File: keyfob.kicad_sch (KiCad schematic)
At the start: 6 parts, among them U1 ATtiny85V-10S

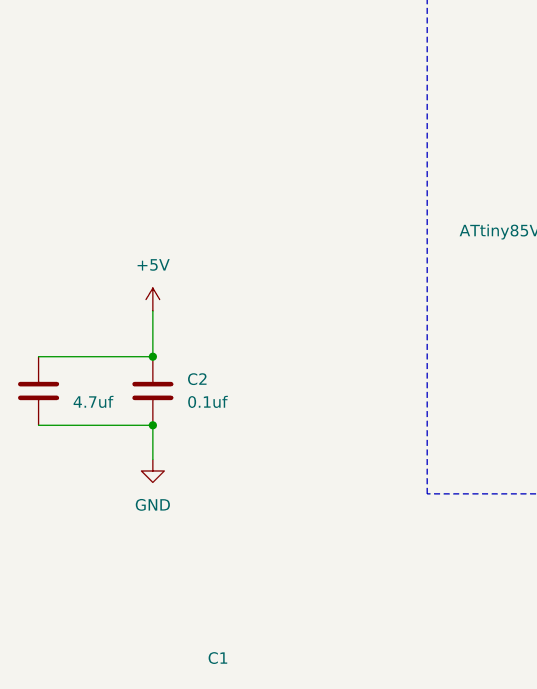
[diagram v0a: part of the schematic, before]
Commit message: Initial commit
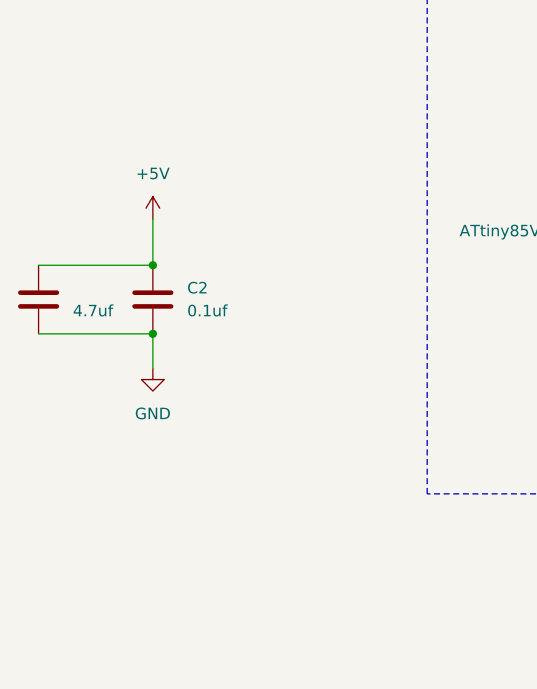
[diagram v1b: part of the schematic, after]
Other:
- moved on the sheet: C2
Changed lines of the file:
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@@
 	(paper "A4")
 	(junction
-		(at 142.24 113.03)
+		(at 142.24 102.87)
 		(diameter 0)
 		(color 0 0 0 0)
 	)
 	(junction
-		(at 142.24 120.65)
+		(at 142.24 110.49)
 		(diameter 0)
 		(color 0 0 0 0)
@@
 	(wire
 		(pts
-			(xy 129.54 113.03) (xy 142.24 113.03)
+			(xy 129.54 102.87) (xy 142.24 102.87)
 		)
 		(stroke
@@
 	(wire
 		(pts
-			(xy 142.24 107.95) (xy 142.24 113.03)
+			(xy 142.24 97.79) (xy 142.24 102.87)
 		)
 		(stroke
@@
 	(wire
 		(pts
-			(xy 129.54 120.65) (xy 142.24 120.65)
+			(xy 129.54 110.49) (xy 142.24 110.49)
 		)
 		(stroke
@@
 	(wire
 		(pts
-			(xy 142.24 120.65) (xy 142.24 124.46)
+			(xy 142.24 110.49) (xy 142.24 114.3)
 		)
 		(stroke
@@
 	(symbol
 		(lib_id "Device:C")
-		(at 129.54 116.84 0)
+		(at 129.54 106.68 0)
 		(unit 1)
 		(exclude_from_sim no)
@@
 		(dnp no)
 		(property "Reference" "C1"
-			(at 148.336 146.558 0)
+			(at 148.844 135.382 0)
 			(effects
 				(font
@@
 				)
 				(justify left)
+				(hide yes)
 			)
 		)
 		(property "Value" "4.7uf"
-			(at 133.35 118.1099 0)
+			(at 133.35 107.9499 0)
 			(effects
 				(font
@@
 		)
 		(property "Footprint" ""
-			(at 130.5052 120.65 0)
+			(at 130.5052 110.49 0)
 			(effects
 				(font
@@
 		)
 		(property "Datasheet" "~"
-			(at 129.54 116.84 0)
+			(at 129.54 106.68 0)
 			(effects
 				(font
@@
 		)
 		(property "Description" "Unpolarized capacitor"
-			(at 129.54 116.84 0)
+			(at 129.54 106.68 0)
 			(effects
 				(font
@@
 	(symbol
 		(lib_id "power:VCC")
-		(at 142.24 107.95 0)
+		(at 142.24 97.79 0)
 		(unit 1)
 		(exclude_from_sim no)
@@
 		(fields_autoplaced yes)
 		(property "Reference" "#PWR01"
-			(at 142.24 111.76 0)
+			(at 142.24 101.6 0)
 			(effects
 				(font
@@
 		)
 		(property "Value" "+5V"
-			(at 142.24 102.87 0)
-			(effects
-				(font
-					(size 1.27 1.27)
-				)
-			)
-		)
-		(property "Footprint" ""
-			(at 142.24 107.95 0)
+			(at 142.24 92.71 0)
+			(effects
+				(font
+					(size 1.27 1.27)
+				)
+			)
+		)
+		(property "Footprint" ""
+			(at 142.24 97.79 0)
 			(effects
 				(font
@@
 		)
 		(property "Datasheet" ""
-			(at 142.24 107.95 0)
+			(at 142.24 97.79 0)
 			(effects
 				(font
@@
 		)
 		(property "Description" "Power symbol creates a global label with name \"VCC\""
-			(at 142.24 107.95 0)
+			(at 142.24 97.79 0)
 			(effects
 				(font
@@
 	(symbol
 		(lib_id "power:GND")
-		(at 142.24 124.46 0)
+		(at 142.24 114.3 0)
 		(unit 1)
 		(exclude_from_sim no)
@@
 		(fields_autoplaced yes)
 		(property "Reference" "#PWR02"
-			(at 142.24 130.81 0)
+			(at 142.24 120.65 0)
 			(effects
 				(font
@@
 		)
 		(property "Value" "GND"
-			(at 142.24 129.54 0)
-			(effects
-				(font
-					(size 1.27 1.27)
-				)
-			)
-		)
-		(property "Footprint" ""
-			(at 142.24 124.46 0)
+			(at 142.24 119.38 0)
+			(effects
+				(font
+					(size 1.27 1.27)
+				)
+			)
+		)
+		(property "Footprint" ""
+			(at 142.24 114.3 0)
 			(effects
 				(font
@@
 		)
 		(property "Datasheet" ""
-			(at 142.24 124.46 0)
+			(at 142.24 114.3 0)
 			(effects
 				(font
@@
 		)
 		(property "Description" "Power symbol creates a global label with name \"GND\" , ground"
-			(at 142.24 124.46 0)
+			(at 142.24 114.3 0)
 			(effects
 				(font
@@
 	(symbol
 		(lib_id "Device:C")
-		(at 142.24 116.84 0)
+		(at 142.24 106.68 0)
 		(unit 1)
 		(exclude_from_sim no)
@@
 		(fields_autoplaced yes)
 		(property "Reference" "C2"
-			(at 146.05 115.5699 0)
+			(at 146.05 105.4099 0)
 			(effects
 				(font
@@
 		)
 		(property "Value" "0.1uf"
-			(at 146.05 118.1099 0)
+			(at 146.05 107.9499 0)
 			(effects
 				(font
@@
 		)
 		(property "Footprint" ""
-			(at 143.2052 120.65 0)
+			(at 143.2052 110.49 0)
 			(effects
 				(font
@@
 		)
 		(property "Datasheet" "~"
-			(at 142.24 116.84 0)
+			(at 142.24 106.68 0)
 			(effects
 				(font
@@
 		)
 		(property "Description" "Unpolarized capacitor"
-			(at 142.24 116.84 0)
-			(effects
-				(font
+			(at 142.24 106.68 0)
+			(effects
+				(font
